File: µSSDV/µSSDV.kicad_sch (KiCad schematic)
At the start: 12 parts, among them J1 Conn_01x02_Pin, U1 ESP32-CAM, U2 atgm336h gps, U3 RFM98W-433S2, U4 TLV61070ADBV

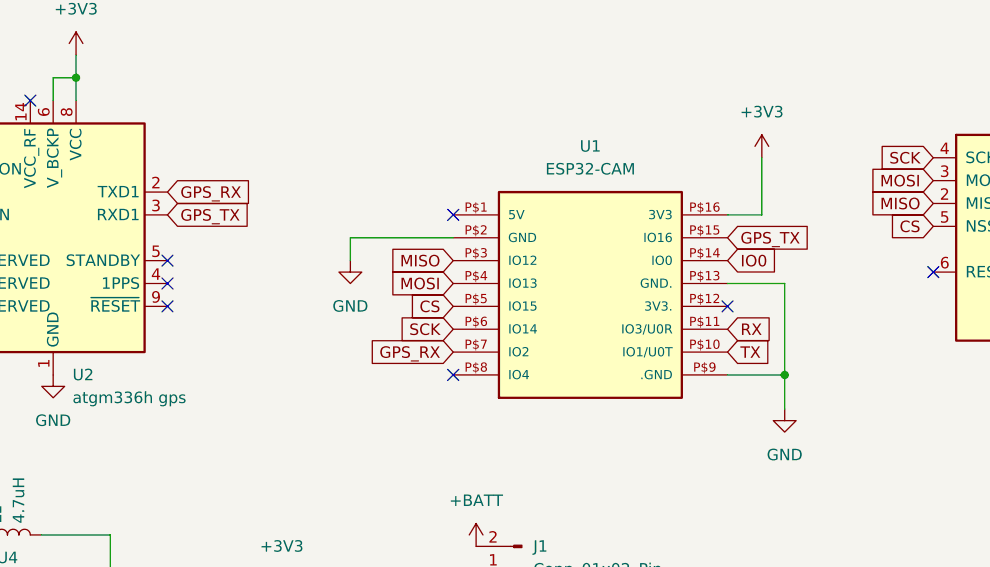
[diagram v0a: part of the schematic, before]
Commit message: Minor PCB updates
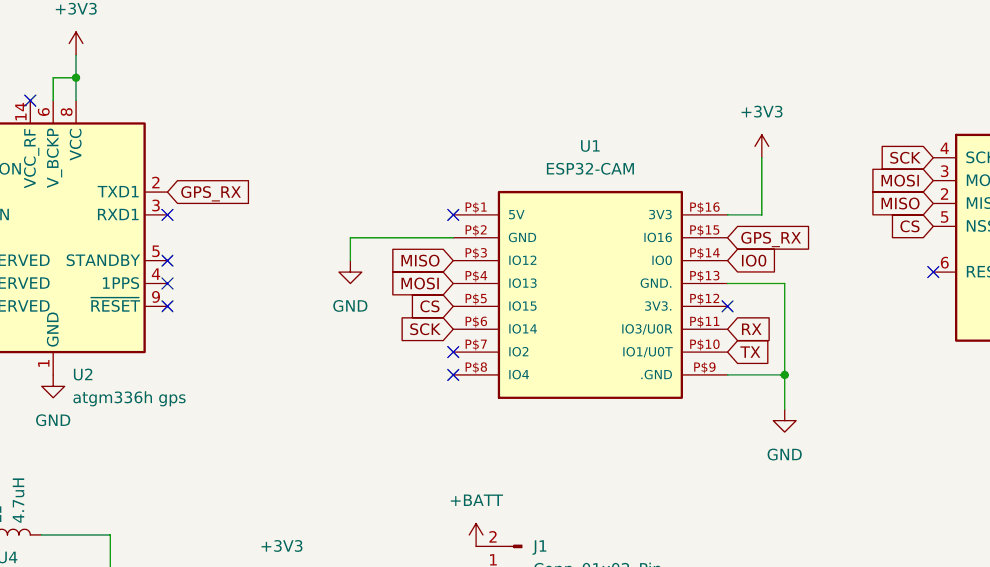
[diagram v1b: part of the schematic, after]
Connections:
- net GPS_RX: now also U1.P$15 (IO16); no longer U1.P$7 (IO2)
- net GPS_TX: no longer names the net of U2.3 (RXD1)
- net GPS_TX: no longer U1.P$15 (IO16)
- no-connect marks 18 -> 20
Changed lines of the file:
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@@
+	)
+	(no_connect
+		(at 63.5 52.07)
 	)
 	(no_connect
@@
 	)
 	(no_connect
+		(at 95.25 67.31)
+	)
+	(no_connect
 		(at 95.25 52.07)
 	)
@@
 		)
 	)
-	(global_label "GPS_TX"
-		(shape input)
-		(at 63.5 52.07 0)
+	(global_label "RX"
+		(shape input)
+		(at 125.73 64.77 0)
 		(fields_autoplaced yes)
 		(effects
@@
 		)
 		(property "Intersheetrefs" "${INTERSHEET_REFS}"
-			(at 73.3794 52.07 0)
+			(at 131.1947 64.77 0)
 			(effects
 				(font
@@
 		)
 	)
-	(global_label "RX"
-		(shape input)
-		(at 125.73 64.77 0)
+	(global_label "GPS_RX"
+		(shape input)
+		(at 125.73 54.61 0)
 		(fields_autoplaced yes)
 		(effects
@@
 		)
 		(property "Intersheetrefs" "${INTERSHEET_REFS}"
-			(at 131.1947 64.77 0)
+			(at 135.9118 54.61 0)
 			(effects
 				(font
@@
 		)
 	)
-	(global_label "GPS_RX"
-		(shape input)
-		(at 95.25 67.31 180)
+	(global_label "CS"
+		(shape input)
+		(at 148.59 53.34 180)
 		(fields_autoplaced yes)
 		(effects
@@
 		)
 		(property "Intersheetrefs" "${INTERSHEET_REFS}"
-			(at 85.0682 67.31 0)
+			(at 143.1253 53.34 0)
 			(effects
 				(font
@@
 		)
 	)
-	(global_label "CS"
-		(shape input)
-		(at 148.59 53.34 180)
+	(global_label "SCK"
+		(shape input)
+		(at 95.25 64.77 180)
 		(fields_autoplaced yes)
 		(effects
@@
 		)
 		(property "Intersheetrefs" "${INTERSHEET_REFS}"
-			(at 143.1253 53.34 0)
+			(at 88.5153 64.77 0)
 			(effects
 				(font
@@
 	(global_label "SCK"
 		(shape input)
-		(at 95.25 64.77 180)
+		(at 148.59 45.72 180)
 		(fields_autoplaced yes)
 		(effects
@@
 		)
 		(property "Intersheetrefs" "${INTERSHEET_REFS}"
-			(at 88.5153 64.77 0)
+			(at 141.8553 45.72 0)
 			(effects
 				(font
@@
 		)
 	)
-	(global_label "SCK"
-		(shape input)
-		(at 148.59 45.72 180)
+	(global_label "IO0"
+		(shape input)
+		(at 125.73 57.15 0)
+		(fields_autoplaced yes)
+		(effects
+			(font
+				(size 1.27 1.27)
+			)
+			(justify left)
+		)
+		(property "Intersheetrefs" "${INTERSHEET_REFS}"
+			(at 131.86 57.15 0)
+			(effects
+				(font
+					(size 1.27 1.27)
+				)
+				(justify left)
+				(hide yes)
+			)
+		)
+	)
+	(global_label "MISO"
+		(shape input)
+		(at 148.59 50.8 180)
 		(fields_autoplaced yes)
 		(effects
@@
 		)
 		(property "Intersheetrefs" "${INTERSHEET_REFS}"
-			(at 141.8553 45.72 0)
+			(at 141.0086 50.8 0)
 			(effects
 				(font
@@
 				(hide yes)
 			)
-		)
-	)
-	(global_label "IO0"
-		(shape input)
-		(at 125.73 57.15 0)
-		(fields_autoplaced yes)
-		(effects
-			(font
-				(size 1.27 1.27)
-			)
-			(justify left)
-		)
-		(property "Intersheetrefs" "${INTERSHEET_REFS}"
-			(at 131.86 57.15 0)
-			(effects
-				(font
-					(size 1.27 1.27)
-				)
-				(justify left)
-				(hide yes)
-			)
-		)
-	)
-	(global_label "MISO"
-		(shape input)
-		(at 148.59 50.8 180)
-		(fields_autoplaced yes)
-		(effects
-			(font
-				(size 1.27 1.27)
-			)
-			(justify right)
-		)
-		(property "Intersheetrefs" "${INTERSHEET_REFS}"
-			(at 141.0086 50.8 0)
-			(effects
-				(font
-					(size 1.27 1.27)
-				)
-				(justify right)
-				(hide yes)
-			)
-		)
-	)
-	(global_label "GPS_TX"
-		(shape input)
-		(at 125.73 54.61 0)
-		(fields_autoplaced yes)
-		(effects
-			(font
-				(size 1.27 1.27)
-			)
-			(justify left)
-		)
-		(property "Intersheetrefs" "${INTERSHEET_REFS}"
-			(at 135.6094 54.61 0)
-			(effects
-				(font
-					(size 1.27 1.27)
-				)
-				(justify left)
-				(hide yes)
-			)
